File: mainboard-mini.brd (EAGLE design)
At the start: 56.8 x 67.3 mm, 105 parts, among them IC1 XC6206P332MR, IC2 LM2901, IC3 NC7SZ10P6X, IC4 STM32F103RBT6, IC5 TDA2822D, IC6 SN65HVD230, IC7 RT8259GE, Q1 8MHz

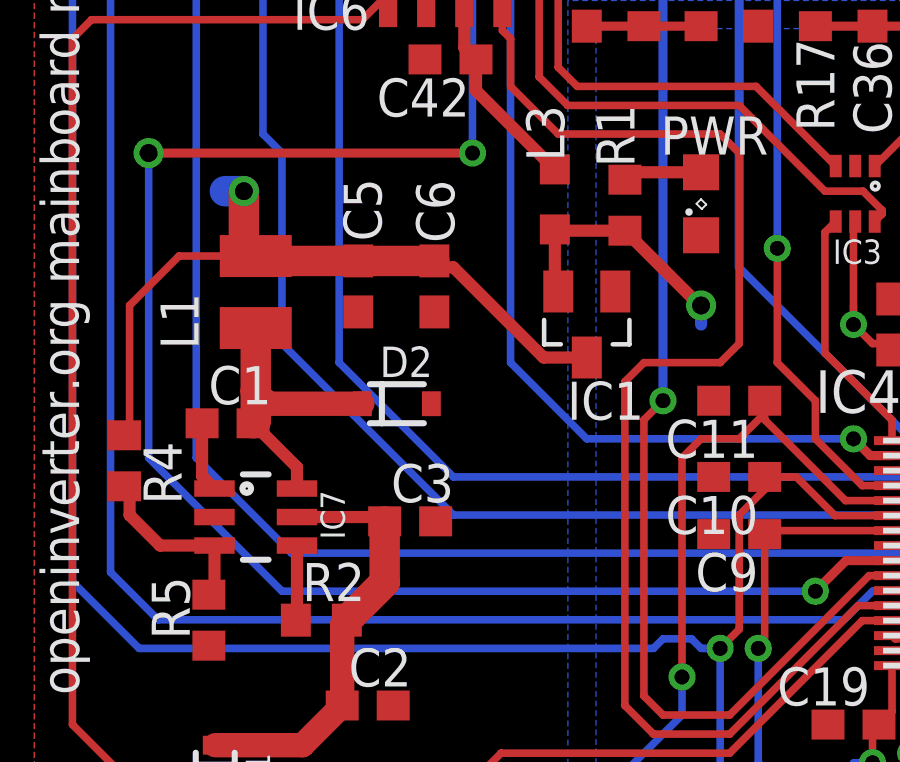
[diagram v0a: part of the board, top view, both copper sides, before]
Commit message: Added new files
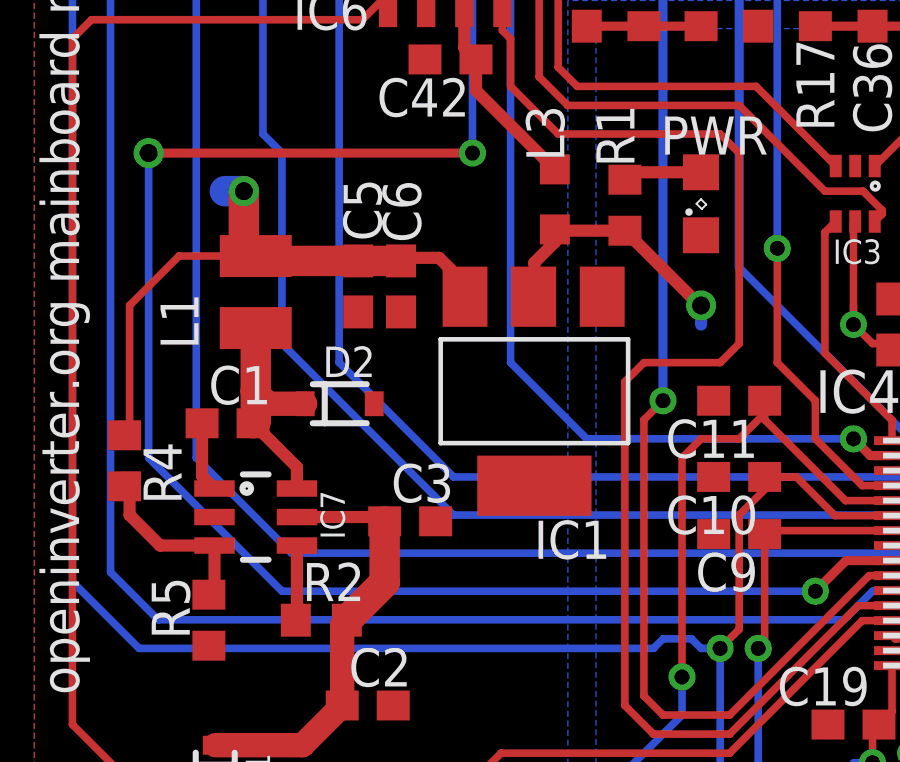
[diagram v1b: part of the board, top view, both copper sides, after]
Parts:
- IC1: device linear:SOT23 -> burr-brown:SOT223
- moved IC1 2.83 mm to (17.9, 33.3)
- moved D2 1.91 mm to (11.4, 32.9)
- moved C6 1.11 mm to (13.5, 36.8)
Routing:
- net VCC: track 52.6 -> 48.0 mm
- net N$14: track 9.72 -> 7.82 mm
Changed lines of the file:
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@@
 </element>
 <element name="C3" library="rcl" package="C0603" value="1µ" x="13.7975" y="29"/>
-<element name="D2" library="SparkFun-DiscreteSemi" package="SOD-323" value="1N5819WS" x="13.355" y="32.92" smashed="yes">
-<attribute name="NAME" x="12.7835" y="33.809" size="1.016" layer="25"/>
-<attribute name="VALUE" value="BAT20JFILM" x="11.196" y="29.491" size="1.27" layer="27"/>
-<attribute name="PROD_ID" value="DIO-11623" x="13.355" y="32.92" size="1.778" layer="27" display="off"/>
+<element name="D2" library="SparkFun-DiscreteSemi" package="SOD-323" value="1N5819WS" x="11.45" y="32.92" smashed="yes">
+<attribute name="NAME" x="10.8785" y="33.809" size="1.016" layer="25"/>
+<attribute name="VALUE" value="BAT20JFILM" x="9.291" y="29.491" size="1.27" layer="27"/>
+<attribute name="PROD_ID" value="DIO-11623" x="11.45" y="32.92" size="1.778" layer="27" display="off"/>
 </element>
 <element name="R10" library="rcl" package="R0603" value="10k" x="52.2325" y="41.6175" smashed="yes" rot="R270">
@@
 </element>
 <element name="L1" library="rcl" package="L2825P" value="4.7µH" x="8.65" y="36.6425" rot="R90"/>
-<element name="C6" library="rcl" package="C0603" value="10µ" x="14.605" y="36.83" smashed="yes" rot="R270">
-<attribute name="NAME" x="14" y="40.3775" size="1.27" layer="25" rot="R270"/>
-<attribute name="VALUE" x="12.065" y="38.1" size="1.27" layer="27" rot="R270"/>
+<element name="C6" library="rcl" package="C0603" value="10µ" x="13.49375" y="36.83" smashed="yes" rot="R270">
+<attribute name="NAME" x="12.88875" y="40.3775" size="1.27" layer="25" rot="R270"/>
+<attribute name="VALUE" x="10.95375" y="38.1" size="1.27" layer="27" rot="R270"/>
 </element>
 <element name="C1" library="rcl" package="C0603" value="22n" x="7.7125" y="32.2675"/>
@@
 <attribute name="VALUE" x="13.462" y="11.811" size="1.27" layer="27"/>
 </element>
-<element name="IC1" library="linear" package="SOT23" value="XC6206P332MR" x="19.685" y="35.56" rot="R180"/>
+<element name="IC1" library="burr-brown" package="SOT223" value="XC6206P332MR" x="17.93875" y="33.3375" rot="R180">
+<attribute name="OC_NEWARK" value="14P6981" x="17.93875" y="33.3375" size="1.778" layer="27" rot="R180" display="off"/>
+<attribute name="MPN" value="REG1117" x="17.93875" y="33.3375" size="1.778" layer="27" rot="R180" display="off"/>
+<attribute name="MF" value="" x="17.93875" y="33.3375" size="1.778" layer="27" rot="R180" display="off"/>
+<attribute name="OC_FARNELL" value="1097566" x="17.93875" y="33.3375" size="1.778" layer="27" rot="R180" display="off"/>
+</element>
 <element name="RN2" library="resistor-net" package="CTS742C083" value="470" x="48.26" y="10.16" rot="R180">
 <attribute name="OC_NEWARK" value="unknown" x="48.26" y="10.16" size="1.778" layer="27" rot="R180" display="off"/>
@@
 <contactref element="RN4" pad="7"/>
 <contactref element="RN4" pad="8"/>
-<contactref element="IC1" pad="1"/>
 <contactref element="C31" pad="2"/>
 <contactref element="C30" pad="2"/>
@@
 <contactref element="C2" pad="2"/>
 <contactref element="R27" pad="1"/>
+<contactref element="IC1" pad="1"/>
+<contactref element="IC1" pad="1"/>
 </signal>
 <signal name="VCC">
@@
 <contactref element="C39" pad="+"/>
 <contactref element="JP2" pad="3"/>
-<contactref element="IC1" pad="3"/>
 <wire x1="8.65" y1="37.8425" x2="8.255" y2="38.2375" width="1.016" layer="1"/>
 <wire x1="8.255" y1="38.2375" x2="8.255" y2="40.005" width="1.016" layer="1"/>
@@
 <wire x1="8.65" y1="37.8425" x2="8.8125" y2="37.68" width="1.016" layer="1"/>
 <wire x1="8.8125" y1="37.68" x2="12.065" y2="37.68" width="1.016" layer="1"/>
-<wire x1="12.065" y1="37.68" x2="14.605" y2="37.68" width="1.016" layer="1"/>
-<wire x1="14.605" y1="37.68" x2="14.82" y2="37.465" width="0.4064" layer="1"/>
-<wire x1="14.82" y1="37.465" x2="15.24" y2="37.465" width="0.4064" layer="1"/>
-<wire x1="15.24" y1="37.465" x2="18.245" y2="34.46" width="0.4064" layer="1"/>
-<wire x1="18.245" y1="34.46" x2="19.685" y2="34.46" width="0.4064" layer="1"/>
+<wire x1="12.065" y1="37.68" x2="13.49375" y2="37.68" width="1.016" layer="1"/>
 <wire x1="52.13" y1="46.99" x2="50.165" y2="46.99" width="0.3048" layer="1"/>
 <via x="50.165" y="46.99" extent="1-16" drill="0.5" shape="octagon"/>
@@
 <wire x1="36.615" y1="52.285" x2="39.275" y2="49.625" width="0.3048" layer="1"/>
 <wire x1="39.275" y1="49.625" x2="39.6025" y2="49.625" width="0.3048" layer="1"/>
+<contactref element="IC1" pad="3"/>
+<wire x1="15.62735" y1="36.4871" x2="15.1511" y2="37.39515" width="0.4064" layer="1"/>
+<wire x1="15.1511" y1="37.39515" x2="14.76375" y2="37.7825" width="0.4064" layer="1"/>
+<wire x1="14.76375" y1="37.7825" x2="13.59625" y2="37.7825" width="0.4064" layer="1"/>
+<wire x1="13.59625" y1="37.7825" x2="13.49375" y2="37.68" width="0.4064" layer="1"/>
 </signal>
 <signal name="PA11/CANRX">
@@
 <wire x1="8.65" y1="32.355" x2="8.65" y2="33.3375" width="1.016" layer="1"/>
 <wire x1="8.65" y1="33.3375" x2="8.65" y2="35.4425" width="1.016" layer="1"/>
-<wire x1="12.205" y1="32.92" x2="9.0675" y2="32.92" width="0.8128" layer="1"/>
+<wire x1="10.3" y1="32.92" x2="9.0675" y2="32.92" width="0.8128" layer="1"/>
 <wire x1="9.0675" y1="32.92" x2="8.65" y2="33.3375" width="0.8128" layer="1"/>
 </signal>
@@
 <contactref element="J1" pad="1"/>
 <contactref element="L3" pad="1"/>
-<contactref element="IC1" pad="2"/>
 <contactref element="R10" pad="2"/>
-<wire x1="18.735" y1="36.66" x2="18.62" y2="36.775" width="0.4064" layer="1"/>
-<wire x1="18.62" y1="36.775" x2="18.62" y2="38.73" width="0.4064" layer="1"/>
-<wire x1="18.62" y1="38.73" x2="18.6625" y2="38.6875" width="0.4064" layer="1"/>
-<wire x1="18.6625" y1="38.6875" x2="20.9575" y2="38.6875" width="0.4064" layer="1"/>
 <wire x1="20.9575" y1="38.6875" x2="23.45" y2="36.195" width="0.4064" layer="1"/>
 <wire x1="23.45" y1="36.195" x2="23.495" y2="36.195" width="0.4064" layer="1"/>
@@
 <wire x1="49.2125" y1="20.6375" x2="49.8475" y2="21.2725" width="0.254" layer="16"/>
 <wire x1="49.8475" y1="21.2725" x2="49.8475" y2="21.9075" width="0.254" layer="16"/>
+<contactref element="IC1" pad="2"/>
+<wire x1="20.9575" y1="38.6875" x2="18.6625" y2="38.6875" width="0.4064" layer="1"/>
+<wire x1="18.6625" y1="38.6875" x2="18.62" y2="38.73" width="0.4064" layer="1"/>
+<wire x1="18.62" y1="38.73" x2="18.62" y2="38.305" width="0.4064" layer="1"/>
+<wire x1="18.62" y1="38.305" x2="17.93875" y2="37.62375" width="0.4064" layer="1"/>
+<wire x1="17.93875" y1="37.62375" x2="17.93875" y2="36.5125" width="0.4064" layer="1"/>
+<wire x1="17.93875" y1="36.5125" x2="17.91335" y2="36.4871" width="0.4064" layer="1"/>
 </signal>
 <signal name="NRST">
